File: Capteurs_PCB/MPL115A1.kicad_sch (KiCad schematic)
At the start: 2 parts, among them U1 MPL115A1

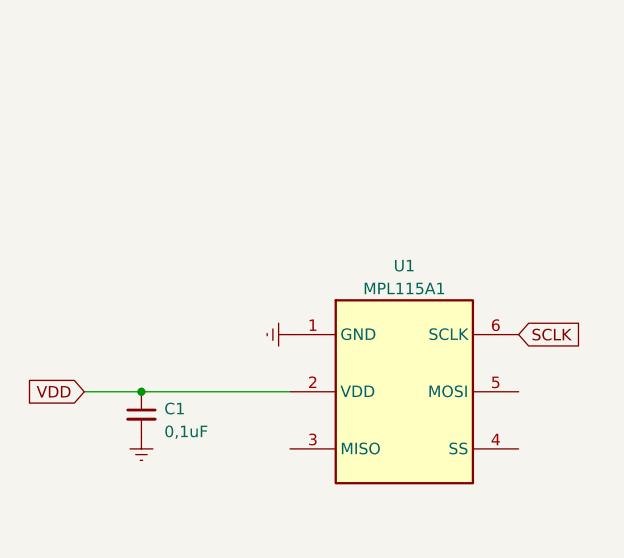
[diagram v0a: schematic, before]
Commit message: pcb update
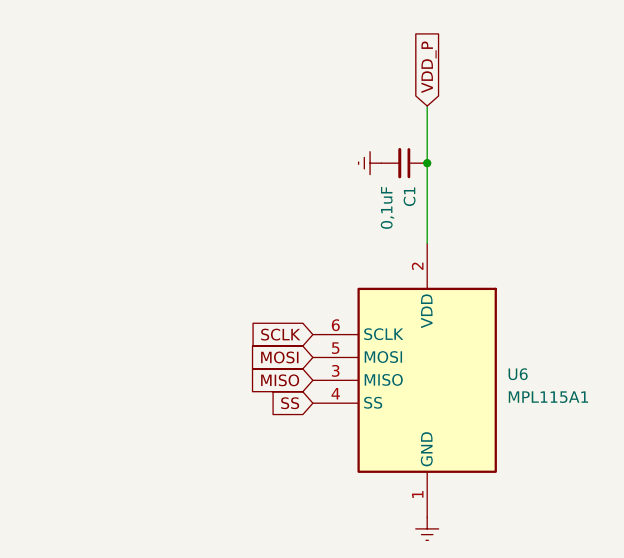
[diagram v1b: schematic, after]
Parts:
- removed U1: MPL115A1, Package_LGA:NXP_LGA-8_3x5mm_P1.25mm_H1.2mm, symbol Sensor_Pressure:MPL115A1
- added U6: MPL115A1, Package_LGA:NXP_LGA-8_3x5mm_P1.25mm_H1.2mm, symbol Sensor_Pressure:MPL115A1
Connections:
- net Earth: now also U6.1 (GND)
- net SCLK: now also U6.6 (SCLK)
- net VDD renamed VDD_P
- net VDD_P: now also U6.2 (VDD)
- new net MISO: U6.3 (MISO)
- new net MOSI: U6.5 (MOSI)
- new net SS: U6.4 (SS)
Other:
- moved on the sheet: C1
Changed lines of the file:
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@@
 (kicad_sch (version 20230121) (generator eeschema)
   (paper "A4")
-  (junction (at 101.6 102.87) (diameter 0) (color 0 0 0 0)
+  (junction (at 133.35 77.47) (diameter 0) (color 0 0 0 0)
   )
-  (wire (pts (xy 95.25 102.87) (xy 101.6 102.87))
+  (wire (pts (xy 133.35 71.12) (xy 133.35 77.47))
     (stroke (width 0) (type default))
   )
-  (wire (pts (xy 101.6 102.87) (xy 118.11 102.87))
+  (wire (pts (xy 133.35 77.47) (xy 133.35 86.36))
     (stroke (width 0) (type default))
   )
-  (global_label "SCLK" (shape input) (at 143.51 96.52 0) (fields_autoplaced)
+  (global_label "MISO" (shape input) (at 120.65 101.6 180) (fields_autoplaced)
+    (effects (font (size 1.27 1.27)) (justify right))
+    (property "Intersheetrefs" "${INTERSHEET_REFS}" (at 113.148 101.6 0)
+      (effects (font (size 1.27 1.27)) (justify right) hide)
+    )
+  )
+  (global_label "SS" (shape input) (at 120.65 104.14 180) (fields_autoplaced)
+    (effects (font (size 1.27 1.27)) (justify right))
+    (property "Intersheetrefs" "${INTERSHEET_REFS}" (at 115.3252 104.14 0)
+      (effects (font (size 1.27 1.27)) (justify right) hide)
+    )
+  )
+  (global_label "SCLK" (shape input) (at 120.65 96.52 180) (fields_autoplaced)
+    (effects (font (size 1.27 1.27)) (justify right))
+    (property "Intersheetrefs" "${INTERSHEET_REFS}" (at 112.9666 96.52 0)
+      (effects (font (size 1.27 1.27)) (justify right) hide)
+    )
+  )
+  (global_label "MOSI" (shape input) (at 120.65 99.06 180) (fields_autoplaced)
+    (effects (font (size 1.27 1.27)) (justify right))
+    (property "Intersheetrefs" "${INTERSHEET_REFS}" (at 113.148 99.06 0)
+      (effects (font (size 1.27 1.27)) (justify right) hide)
+    )
+  )
+  (global_label "VDD_P" (shape input) (at 133.35 71.12 90) (fields_autoplaced)
     (effects (font (size 1.27 1.27)) (justify left))
-    (property "Intersheetrefs" "${INTERSHEET_REFS}" (at 151.1934 96.52 0)
+    (property "Intersheetrefs" "${INTERSHEET_REFS}" (at 133.35 62.348 90)
       (effects (font (size 1.27 1.27)) (justify left) hide)
     )
   )
-  (global_label "VDD" (shape input) (at 95.25 102.87 180) (fields_autoplaced)
-    (effects (font (size 1.27 1.27)) (justify right))
-    (property "Intersheetrefs" "${INTERSHEET_REFS}" (at 88.7156 102.87 0)
-      (effects (font (size 1.27 1.27)) (justify right) hide)
+  (symbol (lib_name "MPL115A1_1") (lib_id "Sensor_Pressure:MPL115A1") (at 133.35 101.6 0) (unit 1)
+    (in_bom yes) (on_board yes) (dnp no) (fields_autoplaced)
+    (property "Reference" "U6" (at 142.24 100.965 0)
+      (effects (font (size 1.27 1.27)) (justify left))
     )
-  )
-  (symbol (lib_id "Sensor_Pressure:MPL115A1") (at 130.81 102.87 90) (unit 1)
-    (in_bom yes) (on_board yes) (dnp no) (fields_autoplaced)
-    (property "Reference" "U1" (at 130.81 88.9 90)
-      (effects (font (size 1.27 1.27)))
+    (property "Value" "MPL115A1" (at 142.24 103.505 0)
+      (effects (font (size 1.27 1.27)) (justify left))
     )
-    (property "Value" "MPL115A1" (at 130.81 91.44 90)
-      (effects (font (size 1.27 1.27)))
-    )
-    (property "Footprint" "Package_LGA:NXP_LGA-8_3x5mm_P1.25mm_H1.2mm" (at 157.48 101.6 0)
+    (property "Footprint" "Package_LGA:NXP_LGA-8_3x5mm_P1.25mm_H1.2mm" (at 134.62 66.04 0)
       (effects (font (size 1.27 1.27)) hide)
     )
-    (property "Datasheet" "http://www.nxp.com/assets/documents/data/en/data-sheets/MPL115A1.pdf" (at 161.29 102.87 0)
+    (property "Datasheet" "http://www.nxp.com/assets/documents/data/en/data-sheets/MPL115A1.pdf" (at 133.35 69.85 0)
       (effects (font (size 1.27 1.27)) hide)
     )
@@
     (instances
       (project "Capteurs_PCB"
-        (path "/1101af8f-9425-4102-9245-339dc54562bf"
-          (reference "U1") (unit 1)
-        )
         (path "/1101af8f-9425-4102-9245-339dc54562bf/3d971057-5943-41d9-af92-399a5cf9d777"
-          (reference "U1") (unit 1)
+          (reference "U6") (unit 1)
         )
       )
     )
   )
-  (symbol (lib_id "power:Earth") (at 101.6 107.95 0) (unit 1)
+  (symbol (lib_id "power:Earth") (at 128.27 77.47 270) (unit 1)
     (in_bom yes) (on_board yes) (dnp no) (fields_autoplaced)
-    (property "Reference" "#PWR01" (at 101.6 114.3 0)
+    (property "Reference" "#PWR01" (at 121.92 77.47 0)
       (effects (font (size 1.27 1.27)) hide)
     )
-    (property "Value" "Earth" (at 101.6 111.76 0)
+    (property "Value" "Earth" (at 124.46 77.47 0)
       (effects (font (size 1.27 1.27)) hide)
     )
-    (property "Footprint" "" (at 101.6 107.95 0)
+    (property "Footprint" "" (at 128.27 77.47 0)
       (effects (font (size 1.27 1.27)) hide)
     )
-    (property "Datasheet" "~" (at 101.6 107.95 0)
+    (property "Datasheet" "~" (at 128.27 77.47 0)
       (effects (font (size 1.27 1.27)) hide)
     )
@@
     )
   )
-  (symbol (lib_id "Device:C_Small") (at 101.6 105.41 0) (unit 1)
+  (symbol (lib_id "Device:C_Small") (at 130.81 77.47 270) (unit 1)
     (in_bom yes) (on_board yes) (dnp no) (fields_autoplaced)
-    (property "Reference" "C1" (at 104.14 104.7813 0)
+    (property "Reference" "C1" (at 131.4387 80.01 0)
       (effects (font (size 1.27 1.27)) (justify left))
     )
-    (property "Value" "0,1uF" (at 104.14 107.3213 0)
+    (property "Value" "0,1uF" (at 128.8987 80.01 0)
       (effects (font (size 1.27 1.27)) (justify left))
     )
-    (property "Footprint" "" (at 101.6 105.41 0)
+    (property "Footprint" "" (at 130.81 77.47 0)
       (effects (font (size 1.27 1.27)) hide)
     )
-    (property "Datasheet" "~" (at 101.6 105.41 0)
+    (property "Datasheet" "~" (at 130.81 77.47 0)
       (effects (font (size 1.27 1.27)) hide)
     )
@@
     )
   )
-  (symbol (lib_id "power:Earth") (at 118.11 96.52 270) (unit 1)
+  (symbol (lib_id "power:Earth") (at 133.35 116.84 0) (unit 1)
     (in_bom yes) (on_board yes) (dnp no) (fields_autoplaced)
-    (property "Reference" "#PWR02" (at 111.76 96.52 0)
+    (property "Reference" "#PWR02" (at 133.35 123.19 0)
       (effects (font (size 1.27 1.27)) hide)
     )
-    (property "Value" "Earth" (at 114.3 96.52 0)
+    (property "Value" "Earth" (at 133.35 120.65 0)
       (effects (font (size 1.27 1.27)) hide)
     )
-    (property "Footprint" "" (at 118.11 96.52 0)
+    (property "Footprint" "" (at 133.35 116.84 0)
       (effects (font (size 1.27 1.27)) hide)
     )
-    (property "Datasheet" "~" (at 118.11 96.52 0)
+    (property "Datasheet" "~" (at 133.35 116.84 0)
       (effects (font (size 1.27 1.27)) hide)
     )
